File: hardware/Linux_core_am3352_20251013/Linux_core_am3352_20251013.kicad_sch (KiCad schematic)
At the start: 0 parts

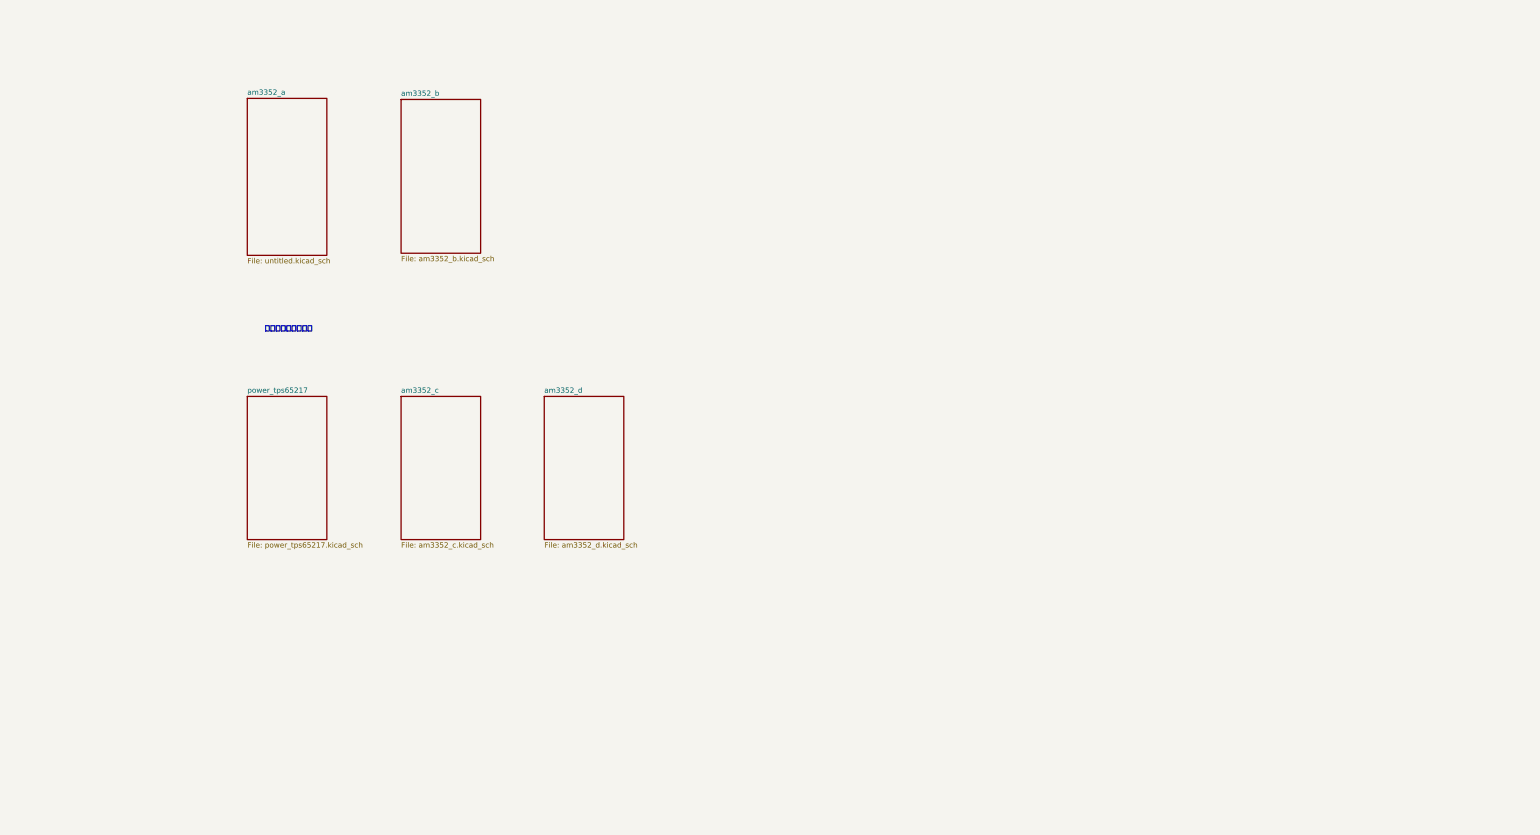
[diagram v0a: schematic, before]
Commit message: update
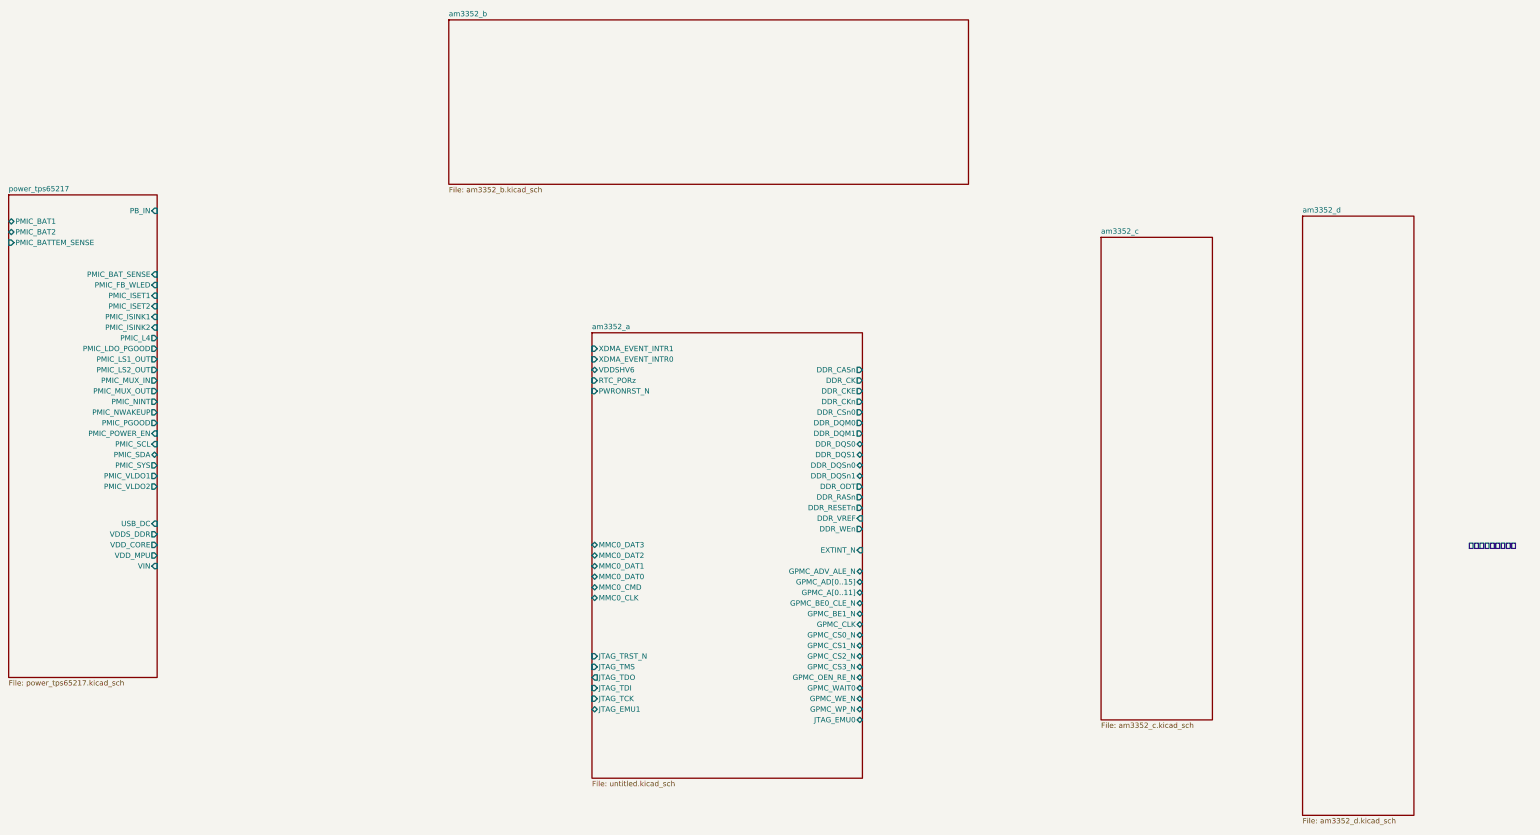
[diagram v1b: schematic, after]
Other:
- sheet am3352_a ports: added DDR_CASn, DDR_CK, DDR_CKE, DDR_CKn, DDR_CSn0, DDR_DQM0, DDR_DQM1, DDR_DQS0, DDR_DQS1, DDR_DQSn0, DDR_DQSn1, DDR_ODT, DDR_RASn, DDR_RESETn, DDR_VREF, DDR_WEn, EXTINT_N, GPMC_ADV_ALE_N, GPMC_AD[0..15], GPMC_A[0..11], GPMC_BE0_CLE_N, GPMC_BE1_N, GPMC_CLK, GPMC_CS0_N, GPMC_CS1_N, GPMC_CS2_N, GPMC_CS3_N, GPMC_OEN_RE_N, GPMC_WAIT0, GPMC_WE_N, GPMC_WP_N, JTAG_EMU0, JTAG_EMU1, JTAG_TCK, JTAG_TDI, JTAG_TDO, JTAG_TMS, JTAG_TRST_N, MMC0_CLK, MMC0_CMD, MMC0_DAT0, MMC0_DAT1, MMC0_DAT2, MMC0_DAT3, PWRONRST_N, RTC_PORz, VDDSHV6, XDMA_EVENT_INTR0, XDMA_EVENT_INTR1; removed none
- sheet power_tps65217 ports: added PB_IN, PMIC_BAT1, PMIC_BAT2, PMIC_BATTEM_SENSE, PMIC_BAT_SENSE, PMIC_FB_WLED, PMIC_ISET1, PMIC_ISET2, PMIC_ISINK1, PMIC_ISINK2, PMIC_L4, PMIC_LDO_PGOOD, PMIC_LS1_OUT, PMIC_LS2_OUT, PMIC_MUX_IN, PMIC_MUX_OUT, PMIC_NINT, PMIC_NWAKEUP, PMIC_PGOOD, PMIC_POWER_EN, PMIC_SCL, PMIC_SDA, PMIC_SYS, PMIC_VLDO1, PMIC_VLDO2, USB_DC, VDDS_DDR, VDD_CORE, VDD_MPU, VIN; removed none
